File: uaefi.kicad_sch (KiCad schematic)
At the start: 67 parts, among them J1 Conn_02x02_Odd_Even, J1 USB_B_Mini, J1 USB_C, J10 5569-16A2, J11 Conn_02x02_Odd_Even, J12 Conn_02x02_Odd_Even, J13 Conn_02x02_Odd_Even, J14 Conn_02x02_Odd_Even, J15 Conn_02x02_Odd_Even, J16 Conn_02x02_Odd_Even, J17 Conn_01x06, J17 Conn_02x02_Odd_Even, J18 Conn_02x02_Odd_Even, J19 Conn_02x02_Odd_Even, J2 5569-20A2, J20 Conn_02x02_Odd_Even, J21 Conn_02x02_Odd_Even, J22 Conn_02x02_Odd_Even, J23 2-6447232-3, J24 Conn_02x02_Odd_Even, J25 2-6447232-3, J3 5569-06A2, J4 5569-08A2, J5 5569-18A2, J5 Conn_01x05_Male, M1 Module-power_12and5V-0.3, M3 Module-knock-0.2, M3 Module-vr-discrete-0.5, M4 Module-vr-max9924-0.1, M5 Module-wbo-0.5, M6 Module:mega-mcu100/0.3, P3 Pad, P4 Pad, P5 Pad, P6 Pad, P7 Pad, P8 Pad, U4 JDY-33

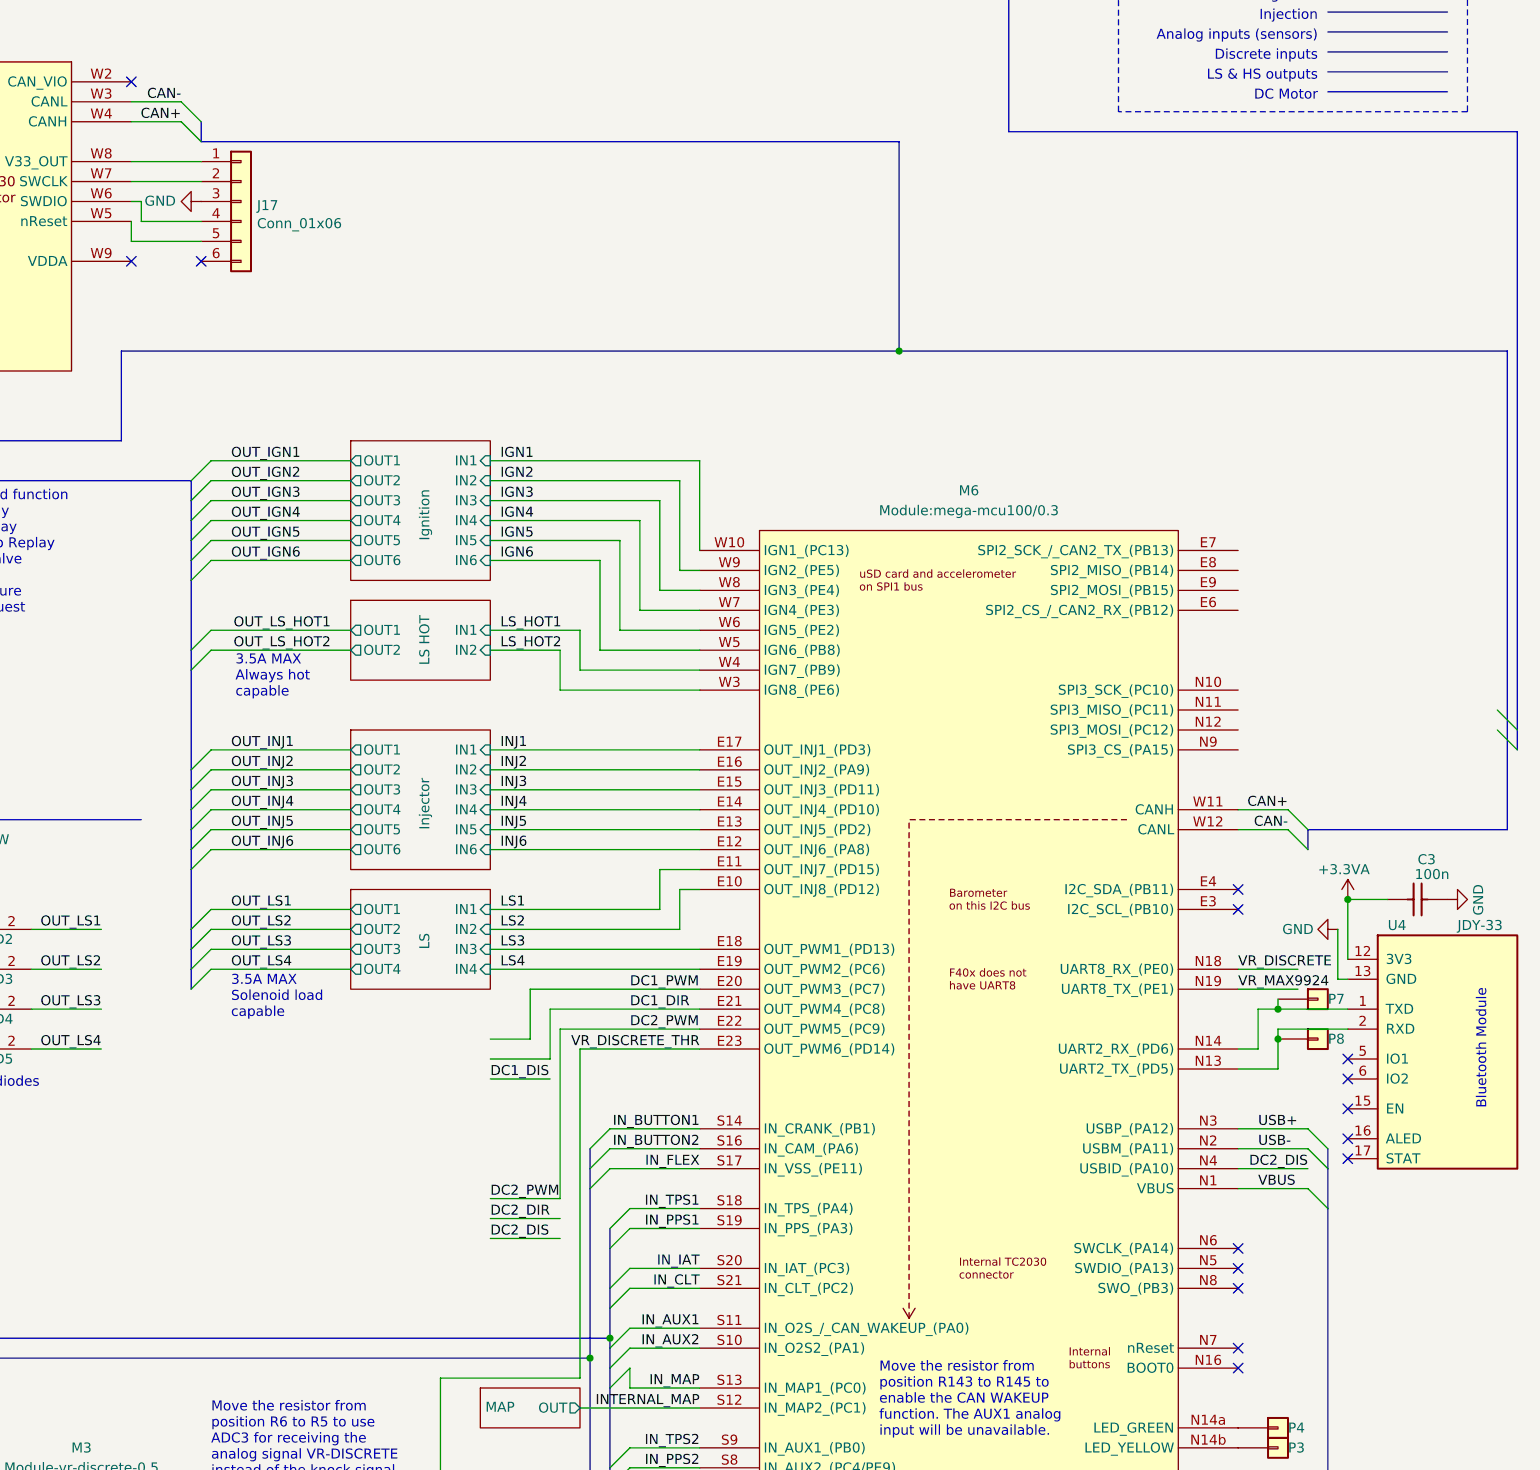
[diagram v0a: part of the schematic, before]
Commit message: a
b
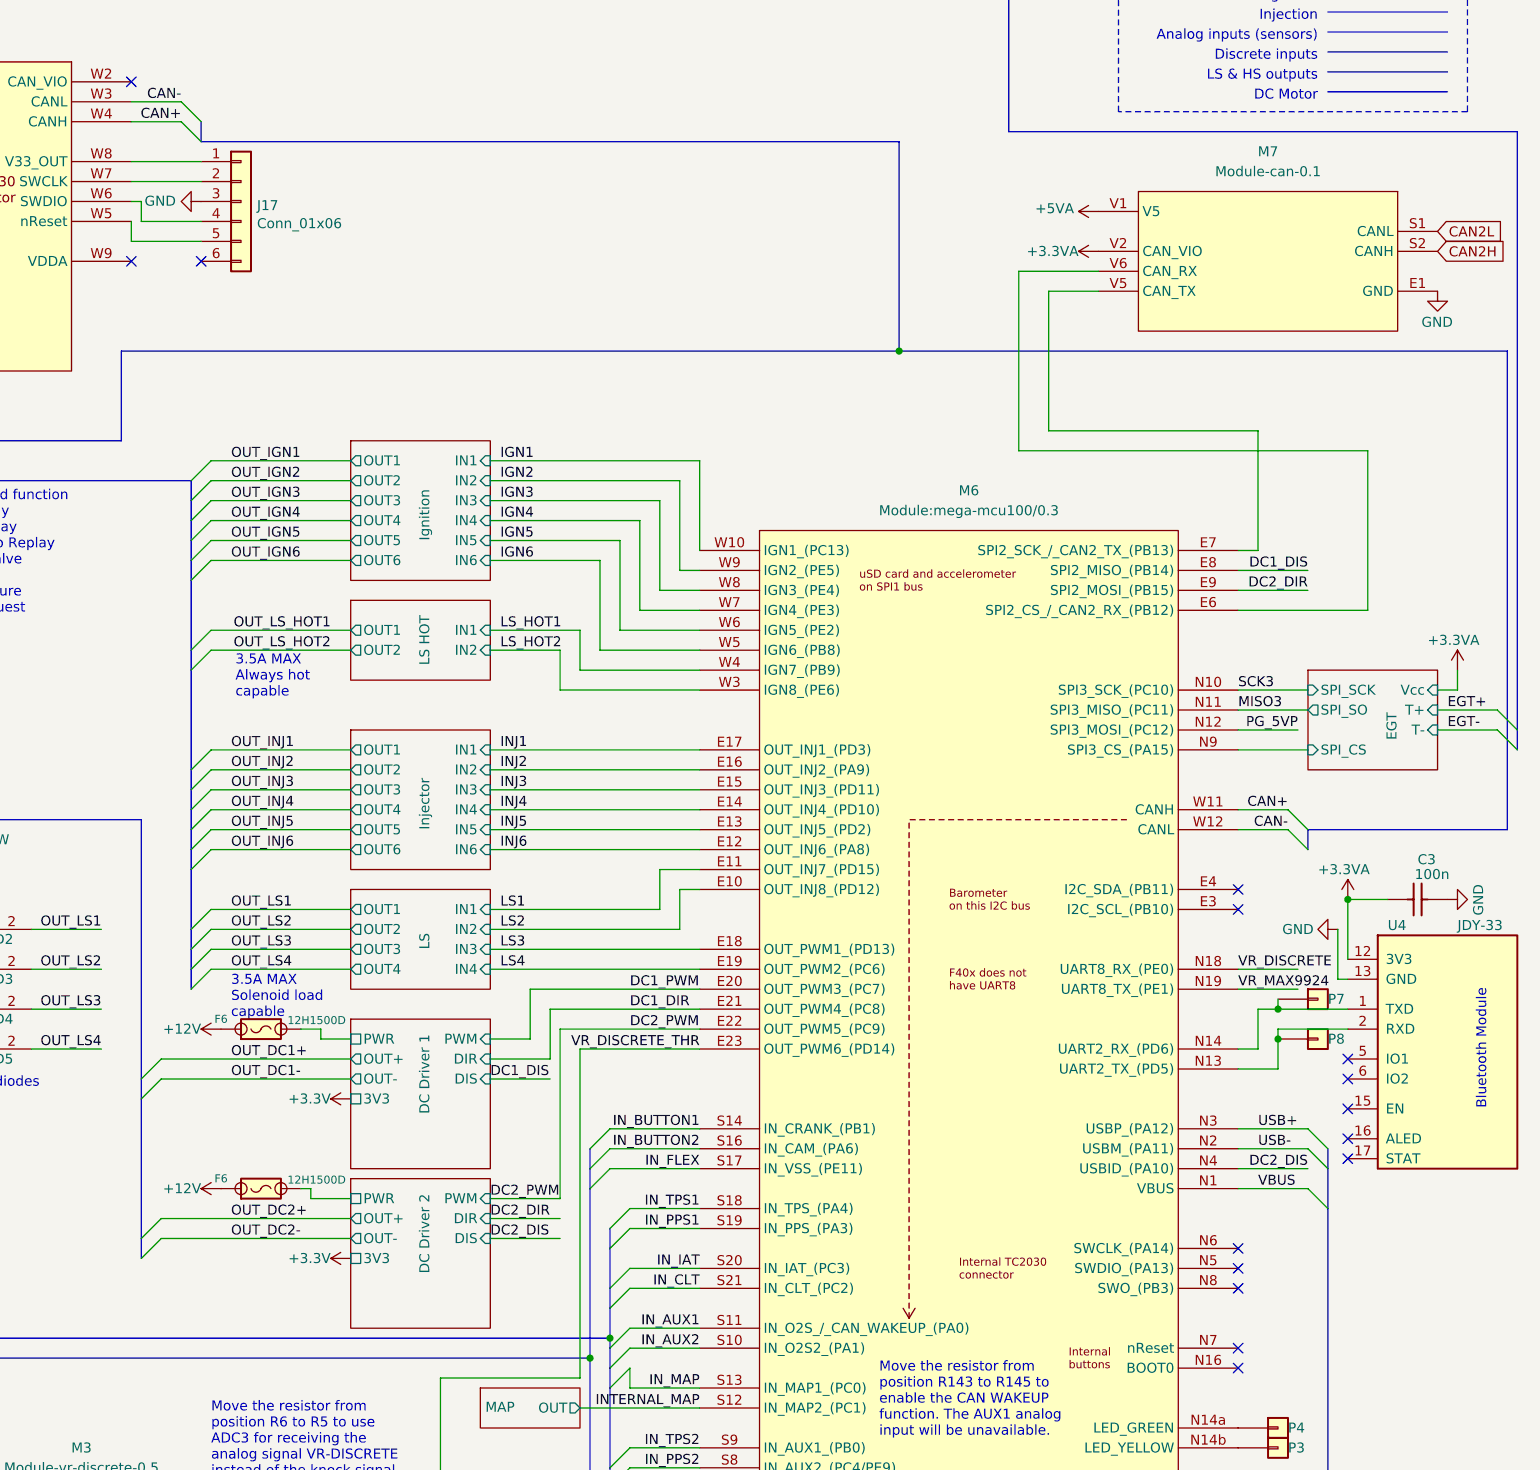
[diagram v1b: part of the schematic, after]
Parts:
- added F6 (x2): 12H1500D, hellen-one-common:PAD-1206-PAD, symbol hellen-one-common:Fuse-Pad-Pad
- added M7: Module-can-0.1, hellen-one-can-0.1:can, symbol hellen-one-can-0.1:Module-can-0.1
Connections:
- net +12V: now also F6.1, F6.1
- net +3.3VA: now also M7.V2 (CAN_VIO)
- net +5VA: now also M7.V1 (V5)
- net CAN2H: now also M7.S2 (CANH)
- net CAN2L: now also M7.S1 (CANL)
- net DC1_DIS: now also M6.E8 (SPI2_MISO_(PB14))
- net DC2_DIR: now also M6.E9 (SPI2_MOSI_(PB15))
- net GND: now also M7.E1 (GND)
- net PG_5VP: now also M6.N12 (SPI3_MOSI_(PC12))
- net at M6.E6 (SPI2_CS_/_CAN2_RX_(PB12)): now also M7.V6 (CAN_RX)
- net at M6.E7 (SPI2_SCK_/_CAN2_TX_(PB13)): now also M7.V5 (CAN_TX)
- net SCK3: now reaches M6.N10 (SPI3_SCK_(PC10))
- net MISO3: now reaches M6.N11 (SPI3_MISO_(PC11))
- net EGT/SPI_CS: now reaches M6.N9 (SPI3_CS_(PA15))
- new net DC Driver 1/PWR: F6.2
- new net DC Driver 2/PWR: F6.2
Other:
- added sheet DC Driver 1 (DC_MOTOR_0.1.kicad_sch)
- added sheet DC Driver 2 (DC_MOTOR_0.1.kicad_sch)
- added sheet EGT (egt.kicad_sch)
